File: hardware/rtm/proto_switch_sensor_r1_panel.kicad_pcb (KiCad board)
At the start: 4 copper layers, 112 x 42 mm, 140 parts, among them IC201 W25Q80, IC202 iCE40HX8K-BG121, IC301 KSZ8081RNA, IC303 MAX5969x, IC402 ECMF04-4HSM10, IC404 ECMF04-4HSM10, IC406 ECMF04-4HSM10, IC408 ECMF04-4HSM10, IC501 TEC 2-4810, IC502 MCP1700, IC503 TEC 2-4815, J202 UART, J302 RJHSE-538x, J401 RJHSE-538x-04, J501 GND, T301 749013011A, X101 M3_MOUNT, X102 M3_MOUNT, X103 M3_MOUNT, X104 M3_MOUNT, Y201 25M, Y301 25M

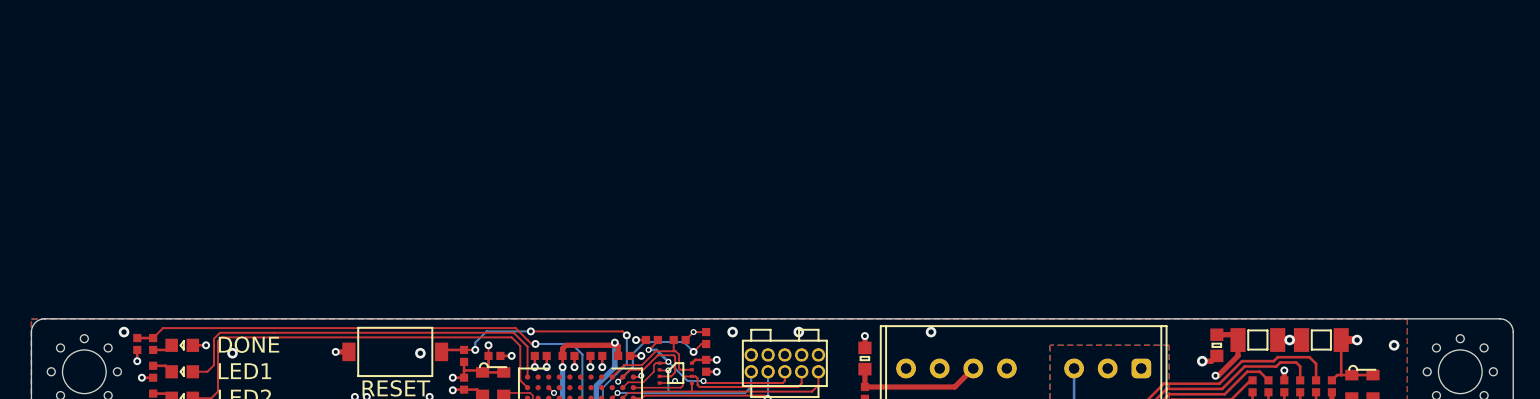
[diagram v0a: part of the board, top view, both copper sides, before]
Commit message: rtm proto sensor and switch
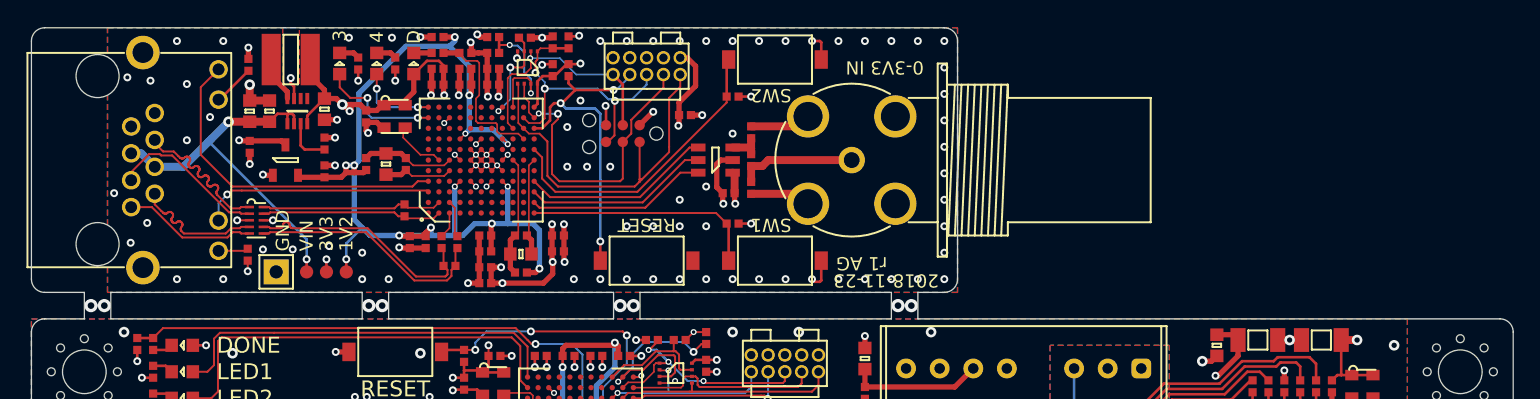
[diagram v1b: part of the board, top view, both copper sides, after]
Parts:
- added C1: 100n, agg:0402, F.Cu at (114.3, 112.9)
- added C10: 10n, agg:0402, F.Cu at (119.8, 111.7)
- added C11: 10n, agg:0402, F.Cu at (114.3, 114.1)
- added C12: 10n, agg:0402, F.Cu at (110.7, 100.3)
- added C13: 10µ, agg:0603, F.Cu at (117.0, 113.1)
- added C14: 100n, agg:0402, F.Cu at (117.0, 111.7)
- added C15: 10µ, agg:0603, F.Cu at (102.2, 102.2)
- added C16: 1µ 48V, agg:0603, F.Cu at (96.5, 102.3)
- added C17: 100n 48V, agg:0603, F.Cu at (98.0, 102.3)
- added C18: 1µ, agg:0402, F.Cu at (102.2, 104.8)
- added C19: 10µ, agg:0603, F.Cu at (106.8, 106.3)
- added C2: 100n, agg:0402, F.Cu at (112.8, 99.1)
- added C20: 100n, agg:0402, F.Cu at (108.3, 106.3)
- added C21: 100n, agg:0402, F.Cu at (96.5, 105.0)
- added C22: 1µ, agg:0402, F.Cu at (102.2, 106.8)
- added C23: 100n, agg:0402, F.Cu at (119.4, 99.2)
- added C24: 100n, agg:0402, F.Cu at (108.6, 112.2)
- added C25: 100n, agg:0402, F.Cu at (132.7, 108.5)
- added C26: 100n, agg:0402, F.Cu at (129.4, 102.6)
- added C27: 10n, agg:0402, F.Cu at (134.4, 103.9)
- added C28: 100n, agg:0402, F.Cu at (105.3, 102.7)
- added C29: 10n, agg:0402, F.Cu at (109.8, 112.2)
- added C3: 10n, agg:0402, F.Cu at (112.8, 100.3)
- added C30: 100n, agg:0402, F.Cu at (110.7, 96.7)
- added C4: 10n, agg:0402, F.Cu at (114.3, 111.7)
- added C5: 100n, agg:0402, F.Cu at (114.3, 115.3)
- added C6: 10n, agg:0402, F.Cu at (114.9, 100.3)
- added C7: 100n, agg:0402, F.Cu at (119.8, 112.9)
- added C8: 100n, agg:0402, F.Cu at (110.7, 99.1)
- added C9: 100n, agg:0402, F.Cu at (114.9, 99.1)
- added D1: LED, agg:0603-LED, F.Cu at (103.3, 98.7)
- added D2: LED, agg:0603-LED, F.Cu at (106.1, 98.7)
- added D3: LED, agg:0603-LED, F.Cu at (108.9, 98.7)
- added D4: ESD_DIODE, agg:0402, F.Cu at (134.4, 108.1)
- added IC1: RJHSE-538x, agg:RJHSE-538X, F.Cu at (85.0, 106.0)
- added IC2: MAX15062, agg:TDFN-8, F.Cu at (100.1, 102.3)
- added IC3: MCP1700, agg:SOT-23, F.Cu at (99.2, 106.0)
- added IC4: iCE40HX8K-BG121, agg:Lattice-BG121, F.Cu at (114.0, 106.0)
- added IC5: W25Q80, agg:UFDFN-8, F.Cu at (117.5, 99.0)
- added IC6: MAX11665AUT, agg:SOT-23-6, F.Cu at (131.7, 106.0)
- added IC7: ECMF04-4HSM10, agg:uQFN-10L, F.Cu at (97.0, 110.5)
- added J1: ~, agg:FTSH-105-01-F-D-K, F.Cu at (126.5, 98.9)
- added J2: ~, agg:TC2030-NL, F.Cu at (124.7, 104.0)
- added J3: GND, agg:SIL-254P-01, F.Cu at (98.5, 114.5)
- added L1: 33µ, agg:LPS4018, F.Cu at (99.6, 98.4)
- added P1: COAX, agg:BNC_PCB_RA_5-1634556-0, F.Cu at (142.0, 106.0)
- added R1: 1k, agg:0402, F.Cu at (96.3, 113.2)
- added R10: 1k, agg:0402, F.Cu at (107.5, 98.7)
- added R11: 1k, agg:0402, F.Cu at (110.7, 97.9)
- added R12: 10k, agg:0402, F.Cu at (120.6, 99.2)
- added R13: 10k, agg:0402, F.Cu at (112.8, 97.9)
- added R14: 10k, agg:0402, F.Cu at (114.9, 97.9)
- added R15: 10k, agg:0402, F.Cu at (117.3, 96.8)
- added R16: 10k, agg:0402, F.Cu at (119.4, 97.1)
- added R17: DNF, agg:0402, F.Cu at (114.9, 96.7)
- added R18: DNF, agg:0402, F.Cu at (120.6, 97.1)
- added R19: 100, agg:0402, F.Cu at (134.4, 106.0)
- added R2: 100, agg:0402, F.Cu at (108.2, 109.8)
- added R20: 10k, agg:0402, F.Cu at (133.0, 101.2)
- added R21: 10k, agg:0402, F.Cu at (133.0, 110.8)
- added R3: 1k, agg:0402, F.Cu at (96.4, 98.8)
- added R4: 140, agg:0402, F.Cu at (112.2, 112.2)
- added R5: 140, agg:0402, F.Cu at (111.6, 114.0)
- added R6: 140, agg:0402, F.Cu at (111.0, 112.2)
- added R7: 100, agg:0402, F.Cu at (117.0, 114.5)
- added R8: 100, agg:0402, F.Cu at (105.3, 106.3)
- added R9: 1k, agg:0402, F.Cu at (104.7, 98.7)
- added SW1: ~, agg:KSR232G, F.Cu at (126.5, 113.6)
- added SW2: ~, agg:KSR232G, F.Cu at (136.2, 98.4)
- added SW3: ~, agg:KSR232G, F.Cu at (136.2, 113.6)
- added TP1: TESTPAD, agg:TESTPAD, F.Cu at (100.8, 114.5)
- added TP2: TESTPAD, agg:TESTPAD, F.Cu at (103.8, 114.5)
- added TP3: TESTPAD, agg:TESTPAD, F.Cu at (102.3, 114.5)
- added Y1: 25M, agg:XTAL-25x20, F.Cu at (107.5, 102.7)
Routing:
- net 1v2: track 68.9 -> 146.0 mm, vias 9 -> 22
- net GND: track 110.0 -> 183.5 mm, vias 100 -> 203
- net 3v3: track 57.5 -> 122.7 mm, vias 28 -> 52
- net /PWRIN: track 0.00 -> 28.7 mm, vias 0 -> 2
- net /FLASH_SDI: track 0.00 -> 28.4 mm
- net /LED2: track 0.00 -> 25.4 mm
- net /CRESET_B: track 0.00 -> 25.3 mm, vias 0 -> 3
- net /FLASH_SCK: track 0.00 -> 24.4 mm, vias 0 -> 2
- net /FLASH_SS: track 0.00 -> 23.1 mm, vias 0 -> 3
- net /USERSW2: track 0.00 -> 22.9 mm
- net /TDESD-: track 0.00 -> 18.3 mm
- net /TDESD+: track 0.00 -> 18.3 mm
- net /FLASH_SDO: track 0.00 -> 18.3 mm, vias 0 -> 1
- net /USERSW1: track 0.00 -> 17.7 mm
- net /LED1: track 0.00 -> 17.6 mm, vias 0 -> 1
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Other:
- board size 112 x 42 mm -> 112 x 64 mm
- net class Default: trace_width 0.15 -> 0.127; via_dia 0.6 -> 0.4572; via_drill 0.3 -> 0.254
- board text added: "0-3V3 IN"
- board text added: "1V2"
- board text added: "2018-11-23"
- board text added: "3"
- board text added: "3V3"
- board text added: "4"
- board text added: "4.5 → 60 VDC IN 4/5: +, 7/8: -"
- board text added: "D"
- board text added: "SW1"
- board text added: "SW2"
- board text added: "VIN"
- board text added: "r1 AG"
